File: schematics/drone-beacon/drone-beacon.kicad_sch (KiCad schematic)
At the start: 14 parts, among them J1 ESP32 Flashing connector, J2 Power Input, SW1 Model selection, U1 ESP32-WROOM-32U, U2 AMS1117-3.3, U3 L96

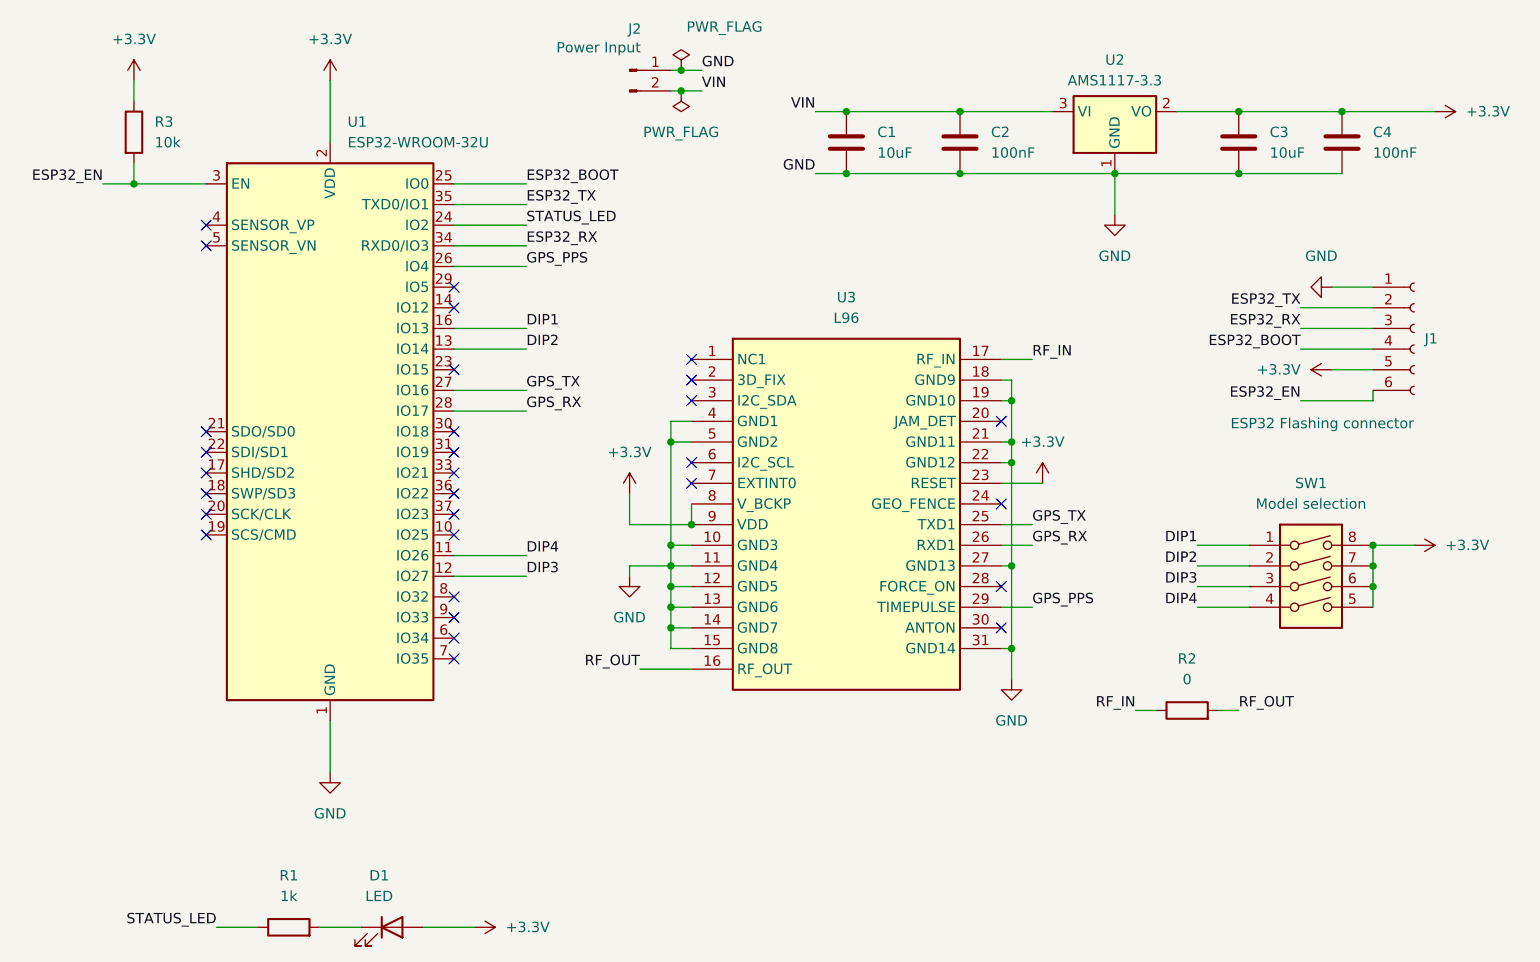
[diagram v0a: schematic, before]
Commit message: Update schematics
Signed-off-by: LAMBS Pierre-Antoine <pierreantoine.lambs@gmail.com>
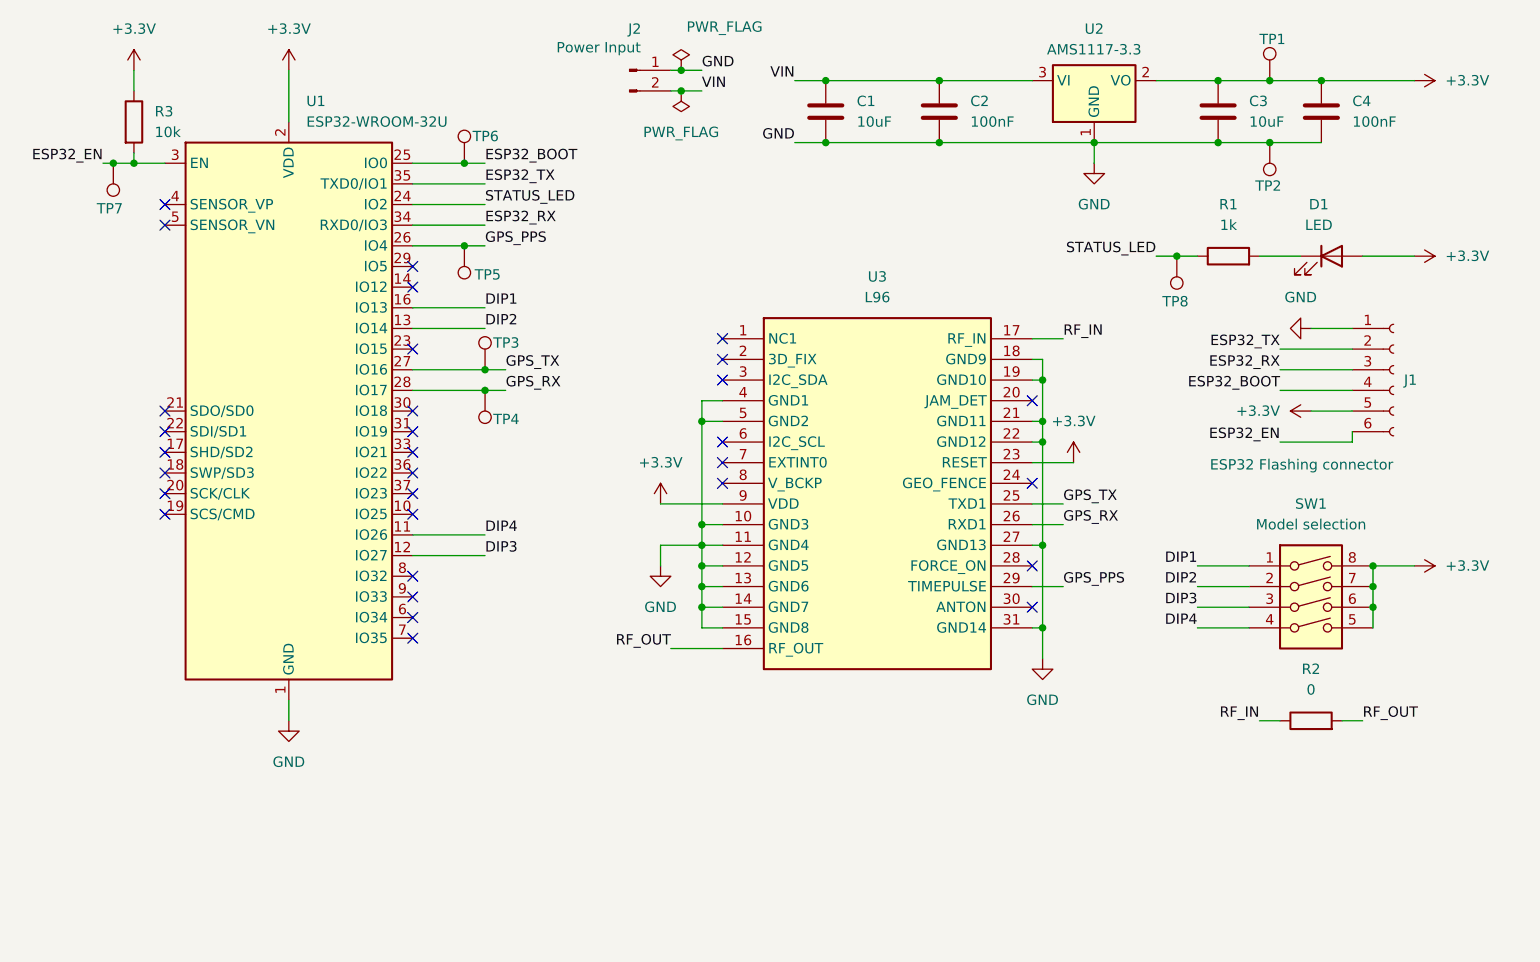
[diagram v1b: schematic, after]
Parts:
- added TP1, TP2, TP3, TP4, TP5, TP6, TP7, TP8: TestPoint, TestPoint:TestPoint_Pad_D1.0mm, symbol Connector:TestPoint
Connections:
- net +3.3V: now also TP1.1; no longer U3.8 (V_BCKP)
- net ESP32_BOOT: now also TP6.1
- net ESP32_EN: now also TP7.1
- net GND: now also TP2.1
- net GPS_PPS: now also TP5.1
- net GPS_RX: now also TP4.1
- net GPS_TX: now also TP3.1
- net STATUS_LED: now also TP8.1
- no-connect marks 30 -> 31
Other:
- moved on the sheet: C1, C2, C3, C4, J1, R1, R2, R3, SW1, U1, U2, U3
